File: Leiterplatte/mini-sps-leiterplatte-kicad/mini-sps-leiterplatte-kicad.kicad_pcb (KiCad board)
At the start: 2 copper layers, 100 x 100 mm, 36 parts, among them J1 Screw_Terminal_01x16, K1 SRD-05VDC-SL-C, K2 SRD-05VDC-SL-C, Q1 BC547, Q2 BC547, U1 L7805

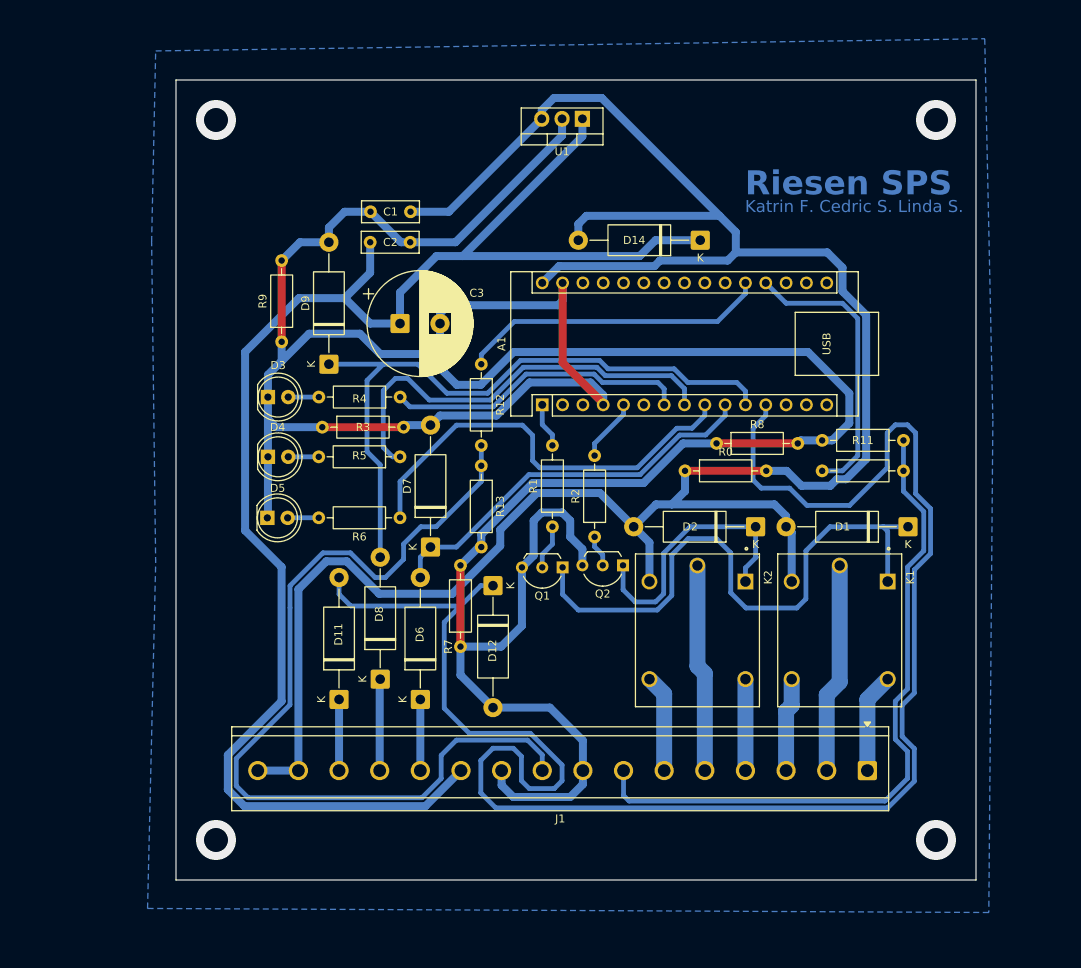
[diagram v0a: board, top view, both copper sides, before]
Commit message: version 2
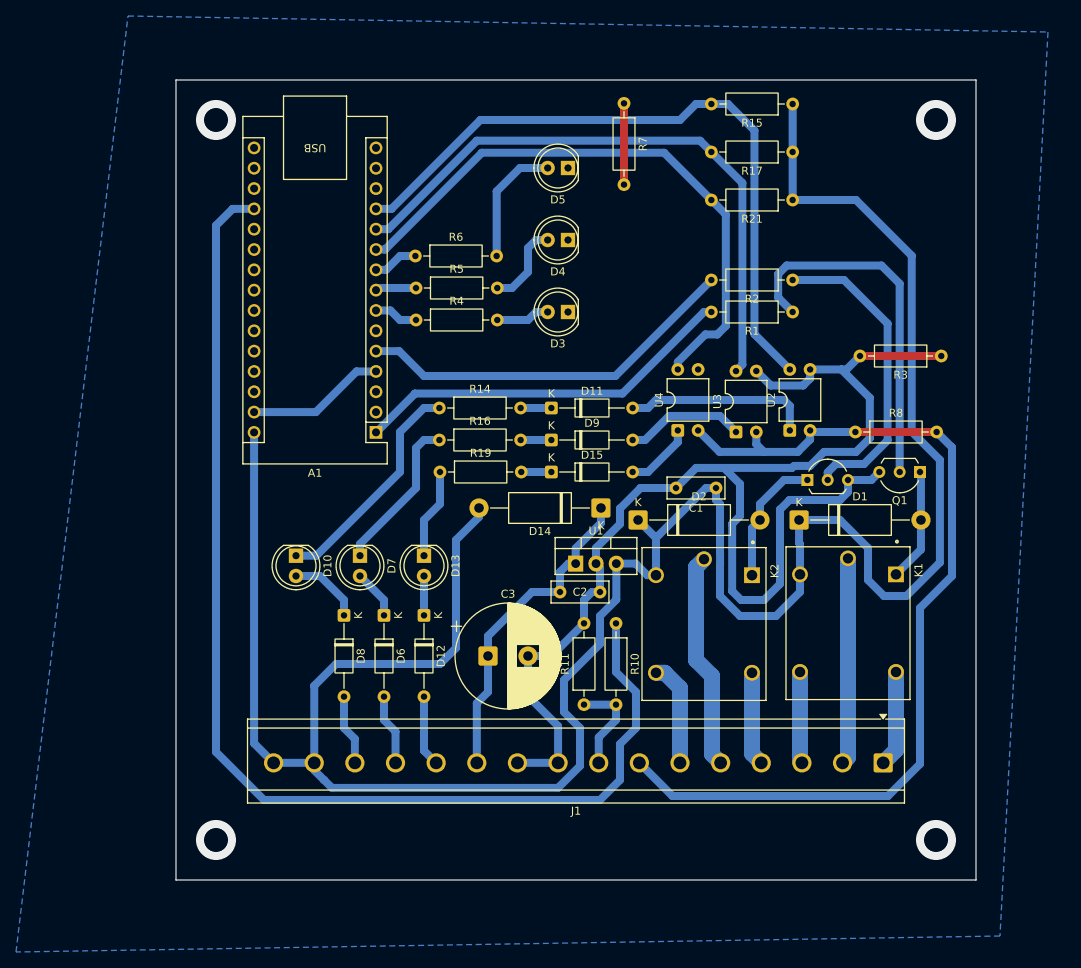
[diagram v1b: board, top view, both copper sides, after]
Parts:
- removed R0, R9: 0, Resistor_THT:R_Axial_DIN0207_L6.3mm_D2.5mm_P10.16mm_Horizontal
- removed R12: 39k, Resistor_THT:R_Axial_DIN0207_L6.3mm_D2.5mm_P10.16mm_Horizontal
- removed R13: 10k, Resistor_THT:R_Axial_DIN0207_L6.3mm_D2.5mm_P10.16mm_Horizontal
- added D10: LED, LED_THT:LED_D5.0mm, F.Cu at (109.5, 111.6)
- added D13: LED, LED_THT:LED_D5.0mm, F.Cu at (125.5, 111.6)
- added D15: BZV55B5V1, Diode_THT:D_DO-35_SOD27_P10.16mm_Horizontal, F.Cu at (141.4, 101.1)
- added R14: 1500, Resistor_THT:R_Axial_DIN0207_L6.3mm_D2.5mm_P10.16mm_Horizontal, F.Cu at (127.4, 93.1)
- added R15: 10k, Resistor_THT:R_Axial_DIN0207_L6.3mm_D2.5mm_P10.16mm_Horizontal, F.Cu at (171.6, 55.1)
- added R16: 1500, Resistor_THT:R_Axial_DIN0207_L6.3mm_D2.5mm_P10.16mm_Horizontal, F.Cu at (127.4, 97.1)
- added R17: 10k, Resistor_THT:R_Axial_DIN0207_L6.3mm_D2.5mm_P10.16mm_Horizontal, F.Cu at (171.6, 61.1)
- added R19: 1500, Resistor_THT:R_Axial_DIN0207_L6.3mm_D2.5mm_P10.16mm_Horizontal, F.Cu at (127.5, 101.1)
- added R21: 10k, Resistor_THT:R_Axial_DIN0207_L6.3mm_D2.5mm_P10.16mm_Horizontal, F.Cu at (171.6, 67.1)
- added U2: PC817, Package_DIP:DIP-4_W7.62mm, F.Cu at (171.2, 95.9)
- added U3: PC817, Package_DIP:DIP-4_W7.62mm, F.Cu at (164.5, 96.1)
- added U4: PC817, Package_DIP:DIP-4_W7.62mm, F.Cu at (157.2, 95.9)
- D11, D9: value D_Zener -> BZV55B5V1; footprint Diode_THT:D_DO-15_P15.24mm_Horizontal -> Diode_THT:D_DO-35_SOD27_P10.16mm_Horizontal
- D12, D6, D8: value D_Zener -> 1N4148WT; footprint Diode_THT:D_DO-15_P15.24mm_Horizontal -> Diode_THT:D_DO-35_SOD27_P10.16mm_Horizontal
- D7: value D_Zener -> LED; footprint Diode_THT:D_DO-15_P15.24mm_Horizontal -> LED_THT:LED_D5.0mm
- K1, K2: footprint custom:RELAY_SRD-05VDC-SL-C -> relay:RELAY_SRD-05VDC-SL-C
- moved R3 77.9 mm to (190.1, 86.6), turned to 180 degrees
- moved R7 70.9 mm to (150.5, 55.0), turned to -90 degrees
- moved D5 57.7 mm to (143.5, 63.1), turned to 180 degrees
- moved U1 55.6 mm to (144.4, 112.6), turned to 0 degrees
- moved R11 51.8 mm to (145.5, 130.2), turned to 90 degrees
- moved C1 51.5 mm to (162.0, 103.1)
- moved C2 49.7 mm to (142.5, 116.1)
- moved D4 46.3 mm to (143.5, 72.1), turned to 180 degrees
- moved Q1 46.2 mm to (187.5, 101.1)
- moved D11 45.1 mm to (141.4, 93.1), turned to 0 degrees
- moved C3 43.0 mm to (133.5, 124.1)
- moved R2 40.5 mm to (171.6, 77.1), turned to 180 degrees
- moved R1 40.3 mm to (171.6, 81.1), turned to 180 degrees
- moved D3 39.0 mm to (143.5, 81.1), turned to 180 degrees
- moved D14 35.7 mm to (147.6, 105.6)
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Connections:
- D1 pad 1: Net-(D1-K) -> +5V
- D1 pad 2: +5V -> Net-(D1-A)
- D11 pad 1: DI3 -> Net-(D11-K)
- D11 pad 2: D9 -> Net-(D11-A)
- D12 pad 1: D9 -> Net-(D12-K)
- D12 pad 2: GND -> DI1
- D2 pad 1: Net-(D2-K) -> +5V
- D2 pad 2: +5V -> Net-(D2-A)
- D6 pad 1: DI1 -> Net-(D6-K)
- D6 pad 2: D7 -> DI2
- D7 pad 1: D7 -> Net-(D7-K)
- D7 pad 2: GND -> Net-(D6-K)
- D8 pad 1: DI2 -> Net-(D10-A)
- D8 pad 2: D8 -> DI3
- D9 pad 1: D8 -> Net-(D9-K)
- D9 pad 2: GND -> Net-(D9-A)
- J1 pad 7: AIN 1 -> GND1
- J1 pad 8: GND -> AIN 1
- J1 pad 9: AIN 2 -> GND
- K1 pad A1: Net-(D1-K) -> Net-(D1-A)
- K2 pad A1: Net-(D2-K) -> Net-(D2-A)
- Q1 pad 1: Net-(D1-K) -> Net-(D1-A)
- Q2 pad 1: Net-(D2-K) -> Net-(D2-A)
- R8 pad 1: GND -> GND1
- R8 pad 2: GND -> GND1
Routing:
- net GND: track 393.9 -> 192.8 mm
- net Vin: track 190.4 -> 41.4 mm
- net D9: track 217.0 -> 85.8 mm
- net GND1: track 0.00 -> 118.1 mm
- net AIN 2: track 111.6 -> 0.00 mm
- net A0: track 35.7 -> 146.9 mm
- net Net-(D1-K): track 75.4 -> 0.00 mm
- net AIN 1: track 85.5 -> 12.2 mm
- net D5(G): track 53.9 -> 5.11 mm
- net D6(B): track 53.7 -> 5.64 mm
- net D1: track 5.61 -> 48.2 mm
- net D2: track 7.85 -> 48.2 mm
- net Net-(Q1-B): track 5.61 -> 45.6 mm
- net A1: track 38.7 -> 0.00 mm
- net Net-(Q2-B): track 3.98 -> 38.8 mm
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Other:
- board text removed: "Katrin F. Cedric S. Linda S."
- board text removed: "Riesen SPS"
